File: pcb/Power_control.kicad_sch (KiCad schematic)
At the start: 3 parts, among them U13 MIC94300

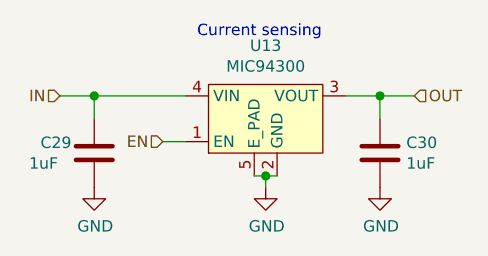
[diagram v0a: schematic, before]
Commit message: Schema: add connections from MCU to voltage measuring circuits
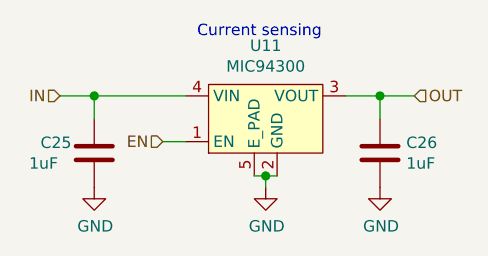
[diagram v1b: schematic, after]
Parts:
- renumbered C29 to C25, C30 to C26, U13 to U11
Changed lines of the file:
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@@
   (symbol (lib_id "power:GND") (at 109.22 97.79 0)
     (in_bom yes) (on_board yes)
-    (property "Reference" "#PWR093" (id 0) (at 109.22 104.14 0)
+    (property "Reference" "#PWR080" (id 0) (at 109.22 104.14 0)
       (effects (font (size 1.27 1.27)) hide)
     )
@@
   (symbol (lib_id "power:GND") (at 128.27 97.79 0)
     (in_bom yes) (on_board yes)
-    (property "Reference" "#PWR094" (id 0) (at 128.27 104.14 0)
+    (property "Reference" "#PWR081" (id 0) (at 128.27 104.14 0)
       (effects (font (size 1.27 1.27)) hide)
     )
@@
   (symbol (lib_id "power:GND") (at 140.97 97.79 0)
     (in_bom yes) (on_board yes)
-    (property "Reference" "#PWR095" (id 0) (at 140.97 104.14 0)
+    (property "Reference" "#PWR082" (id 0) (at 140.97 104.14 0)
       (effects (font (size 1.27 1.27)) hide)
     )
@@
   (symbol (lib_id "Device:C") (at 109.22 93.98 0)
     (in_bom yes) (on_board yes)
-    (property "Reference" "C29" (id 0) (at 103.2511 92.8306 0)
+    (property "Reference" "C25" (id 0) (at 103.2511 92.8306 0)
       (effects (font (size 1.27 1.27)) (justify left))
     )
@@
   (symbol (lib_id "Device:C") (at 140.97 93.98 0)
     (in_bom yes) (on_board yes)
-    (property "Reference" "C30" (id 0) (at 143.8911 92.8306 0)
+    (property "Reference" "C26" (id 0) (at 143.8911 92.8306 0)
       (effects (font (size 1.27 1.27)) (justify left))
     )
@@
   (symbol (lib_id "TCY_IC:MIC94300") (at 128.27 90.17 0)
     (in_bom yes) (on_board yes)
-    (property "Reference" "U13" (id 0) (at 128.27 82.0482 0))
+    (property "Reference" "U11" (id 0) (at 128.27 82.0482 0))
     (property "Value" "MIC94300" (id 1) (at 128.27 84.3469 0))
     (property "Footprint" "TCY_IC:MLF-4_1.2x1.6mm_P0.5_1EP_0.85x0.5mm" (id 2) (at 124.46 90.17 0)

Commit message: Schema: update connection of CS_EN pin
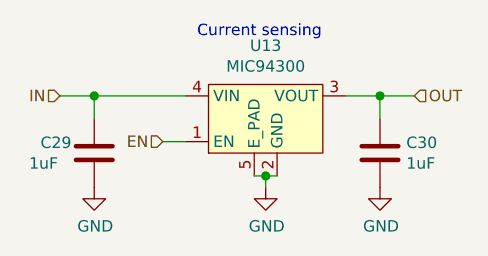
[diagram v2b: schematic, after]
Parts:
- renumbered C25 to C29, C26 to C30, U11 to U13
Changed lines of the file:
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@@
   (symbol (lib_id "power:GND") (at 109.22 97.79 0)
     (in_bom yes) (on_board yes)
-    (property "Reference" "#PWR080" (id 0) (at 109.22 104.14 0)
+    (property "Reference" "#PWR093" (id 0) (at 109.22 104.14 0)
       (effects (font (size 1.27 1.27)) hide)
     )
@@
   (symbol (lib_id "power:GND") (at 128.27 97.79 0)
     (in_bom yes) (on_board yes)
-    (property "Reference" "#PWR081" (id 0) (at 128.27 104.14 0)
+    (property "Reference" "#PWR094" (id 0) (at 128.27 104.14 0)
       (effects (font (size 1.27 1.27)) hide)
     )
@@
   (symbol (lib_id "power:GND") (at 140.97 97.79 0)
     (in_bom yes) (on_board yes)
-    (property "Reference" "#PWR082" (id 0) (at 140.97 104.14 0)
+    (property "Reference" "#PWR095" (id 0) (at 140.97 104.14 0)
       (effects (font (size 1.27 1.27)) hide)
     )
@@
   (symbol (lib_id "Device:C") (at 109.22 93.98 0)
     (in_bom yes) (on_board yes)
-    (property "Reference" "C25" (id 0) (at 103.2511 92.8306 0)
+    (property "Reference" "C29" (id 0) (at 103.2511 92.8306 0)
       (effects (font (size 1.27 1.27)) (justify left))
     )
@@
   (symbol (lib_id "Device:C") (at 140.97 93.98 0)
     (in_bom yes) (on_board yes)
-    (property "Reference" "C26" (id 0) (at 143.8911 92.8306 0)
+    (property "Reference" "C30" (id 0) (at 143.8911 92.8306 0)
       (effects (font (size 1.27 1.27)) (justify left))
     )
@@
   (symbol (lib_id "TCY_IC:MIC94300") (at 128.27 90.17 0)
     (in_bom yes) (on_board yes)
-    (property "Reference" "U11" (id 0) (at 128.27 82.0482 0))
+    (property "Reference" "U13" (id 0) (at 128.27 82.0482 0))
     (property "Value" "MIC94300" (id 1) (at 128.27 84.3469 0))
     (property "Footprint" "TCY_IC:MLF-4_1.2x1.6mm_P0.5_1EP_0.85x0.5mm" (id 2) (at 124.46 90.17 0)

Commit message: Schema: bom optimization
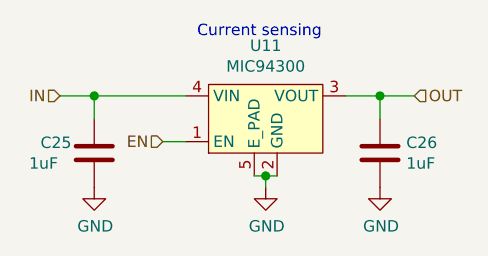
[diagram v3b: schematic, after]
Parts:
- renumbered C29 to C25, C30 to C26, U13 to U11
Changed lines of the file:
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@@
   (symbol (lib_id "Device:C") (at 109.22 93.98 0)
     (in_bom yes) (on_board yes)
-    (property "Reference" "C29" (id 0) (at 103.2511 92.8306 0)
+    (property "Reference" "C25" (id 0) (at 103.2511 92.8306 0)
       (effects (font (size 1.27 1.27)) (justify left))
     )
@@
   (symbol (lib_id "Device:C") (at 140.97 93.98 0)
     (in_bom yes) (on_board yes)
-    (property "Reference" "C30" (id 0) (at 143.8911 92.8306 0)
+    (property "Reference" "C26" (id 0) (at 143.8911 92.8306 0)
       (effects (font (size 1.27 1.27)) (justify left))
     )
@@
   (symbol (lib_id "TCY_IC:MIC94300") (at 128.27 90.17 0)
     (in_bom yes) (on_board yes)
-    (property "Reference" "U13" (id 0) (at 128.27 82.0482 0))
+    (property "Reference" "U11" (id 0) (at 128.27 82.0482 0))
     (property "Value" "MIC94300" (id 1) (at 128.27 84.3469 0))
     (property "Footprint" "TCY_IC:MLF-4_1.2x1.6mm_P0.5_1EP_0.85x0.5mm" (id 2) (at 124.46 90.17 0)

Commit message: Schema: update footprint 3-pin connectors, project cleanup, add gitignore
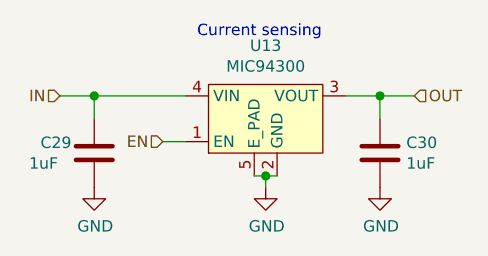
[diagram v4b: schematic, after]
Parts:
- renumbered C25 to C29, C26 to C30, U11 to U13
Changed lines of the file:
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@@
   (symbol (lib_id "Device:C") (at 109.22 93.98 0)
     (in_bom yes) (on_board yes)
-    (property "Reference" "C25" (id 0) (at 103.2511 92.8306 0)
+    (property "Reference" "C29" (id 0) (at 103.2511 92.8306 0)
       (effects (font (size 1.27 1.27)) (justify left))
     )
@@
   (symbol (lib_id "Device:C") (at 140.97 93.98 0)
     (in_bom yes) (on_board yes)
-    (property "Reference" "C26" (id 0) (at 143.8911 92.8306 0)
+    (property "Reference" "C30" (id 0) (at 143.8911 92.8306 0)
       (effects (font (size 1.27 1.27)) (justify left))
     )
@@
   (symbol (lib_id "TCY_IC:MIC94300") (at 128.27 90.17 0)
     (in_bom yes) (on_board yes)
-    (property "Reference" "U11" (id 0) (at 128.27 82.0482 0))
+    (property "Reference" "U13" (id 0) (at 128.27 82.0482 0))
     (property "Value" "MIC94300" (id 1) (at 128.27 84.3469 0))
     (property "Footprint" "TCY_IC:MLF-4_1.2x1.6mm_P0.5_1EP_0.85x0.5mm" (id 2) (at 124.46 90.17 0)
